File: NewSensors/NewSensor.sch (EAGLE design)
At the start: 9 parts, among them X2 CNY70

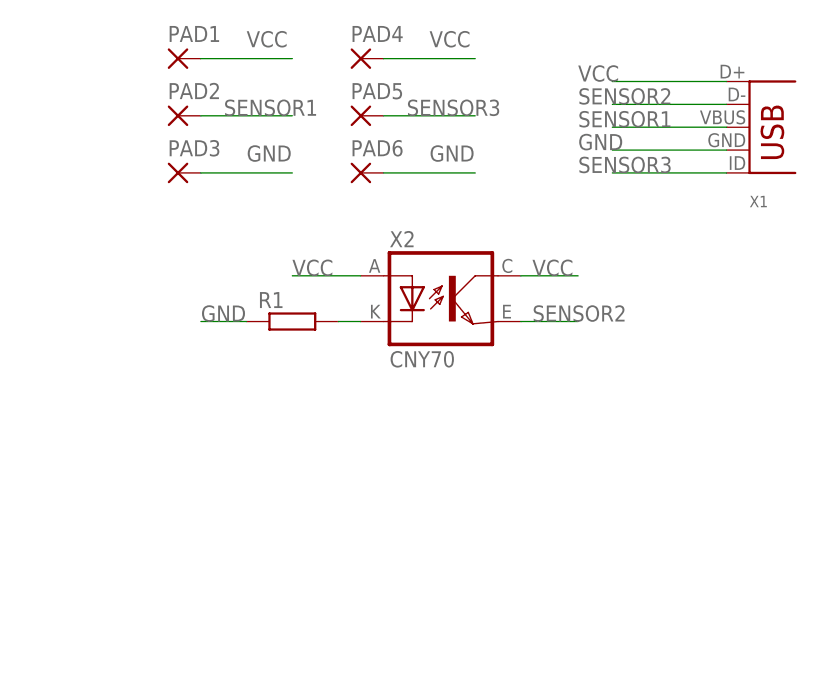
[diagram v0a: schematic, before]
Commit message: Added code V1
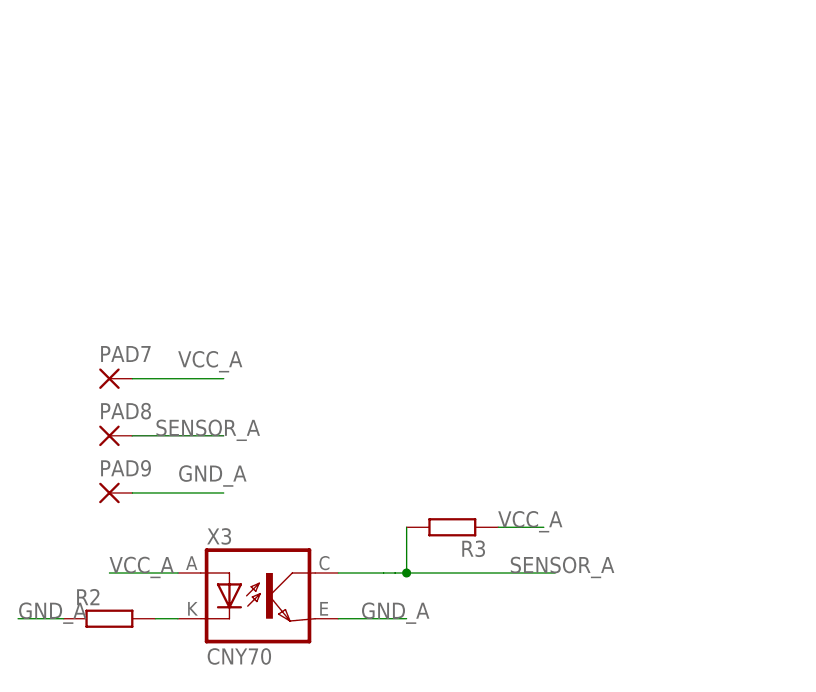
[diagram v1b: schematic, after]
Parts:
- removed PAD1, PAD2, PAD3, PAD4, PAD5, PAD6: WIREPADSMD1,27-254, wirepad:WIREPADSMD1,27-254
- removed R1: (no value), ScyllAlarmV3.0:RCL_R-EU_R0805
- removed X1: (no value), tom:USB-MB-S
- removed X2: CNY70, cny70:CNY70
- added PAD7, PAD8, PAD9: WIREPADSMD1,27-254, wirepad:WIREPADSMD1,27-254
- added R2, R3: (no value), ScyllAlarmV3.0:RCL_R-EU_R0805
- added X3: CNY70, cny70:CNY70
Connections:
- removed net GND: PAD3.P, PAD6.P, R1.1, X1.GND
- removed net N$1: R1.2, X2.C
- removed net SENSOR1: PAD2.P, X1.VBUS
- removed net SENSOR2: X1.D-, X2.EMI
- removed net SENSOR3: PAD5.P, X1.ID
- removed net VCC: PAD1.P, PAD4.P, X1.D+, X2.A, X2.COL
- new net GND_A: PAD9.P, R2.1, X3.EMI
- new net N$2: R2.2, X3.C
- new net SENSOR_A: PAD8.P, R3.2, X3.COL
- new net VCC_A: PAD7.P, R3.1, X3.A
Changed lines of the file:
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@@
 <settings>
 <setting alwaysvectorfont="no"/>
-<setting keepoldvectorfont="yes"/>
 <setting verticaltext="up"/>
 </settings>
@@
 <layer number="88" name="SimResults" color="9" fill="1" visible="yes" active="yes"/>
 <layer number="89" name="SimProbes" color="9" fill="1" visible="yes" active="yes"/>
-<layer number="90" name="Modules" color="5" fill="1" visible="no" active="yes"/>
+<layer number="90" name="Modules" color="5" fill="1" visible="yes" active="yes"/>
 <layer number="91" name="Nets" color="2" fill="1" visible="yes" active="yes"/>
 <layer number="92" name="Busses" color="1" fill="1" visible="yes" active="yes"/>
@@
 </classes>
 <parts>
-<part name="R1" library="ScyllAlarmV3.0" deviceset="RCL_R-EU_" device="R0805"/>
-<part name="X1" library="tom" deviceset="USB" device="-MB-S"/>
-<part name="X2" library="cny70" deviceset="CNY70" device=""/>
-<part name="PAD1" library="wirepad" library_urn="urn:adsk.eagle:library:412" deviceset="WIREPAD" device="SMD1,27-254" package3d_urn="urn:adsk.eagle:package:30839/1" value="WIREPADSMD1,27-254"/>
-<part name="PAD2" library="wirepad" deviceset="WIREPAD" device="SMD1,27-254" value="WIREPADSMD1,27-254"/>
-<part name="PAD3" library="wirepad" deviceset="WIREPAD" device="SMD1,27-254" value="WIREPADSMD1,27-254"/>
-<part name="PAD4" library="wirepad" deviceset="WIREPAD" device="SMD1,27-254" value="WIREPADSMD1,27-254"/>
-<part name="PAD5" library="wirepad" deviceset="WIREPAD" device="SMD1,27-254" value="WIREPADSMD1,27-254"/>
-<part name="PAD6" library="wirepad" deviceset="WIREPAD" device="SMD1,27-254" value="WIREPADSMD1,27-254"/>
+<part name="R2" library="ScyllAlarmV3.0" deviceset="RCL_R-EU_" device="R0805"/>
+<part name="X3" library="cny70" deviceset="CNY70" device=""/>
+<part name="PAD7" library="wirepad" library_urn="urn:adsk.eagle:library:412" deviceset="WIREPAD" device="SMD1,27-254" package3d_urn="urn:adsk.eagle:package:30839/1" value="WIREPADSMD1,27-254"/>
+<part name="PAD8" library="wirepad" deviceset="WIREPAD" device="SMD1,27-254" value="WIREPADSMD1,27-254"/>
+<part name="PAD9" library="wirepad" deviceset="WIREPAD" device="SMD1,27-254" value="WIREPADSMD1,27-254"/>
+<part name="R3" library="ScyllAlarmV3.0" deviceset="RCL_R-EU_" device="R0805"/>
 </parts>
 <sheets>
@@
 </plain>
 <instances>
-<instance part="R1" gate="G$1" x="38.1" y="60.96"/>
-<instance part="X1" gate="G$1" x="88.9" y="78.74"/>
-<instance part="X2" gate="G$1" x="55.88" y="63.5"/>
-<instance part="PAD1" gate="G$1" x="25.4" y="90.17" smashed="yes">
-<attribute name="NAME" x="24.257" y="92.0242" size="1.778" layer="95"/>
+<instance part="R2" gate="G$1" x="17.78" y="27.94"/>
+<instance part="X3" gate="G$1" x="35.56" y="30.48"/>
+<instance part="PAD7" gate="G$1" x="17.78" y="54.61" smashed="yes">
+<attribute name="NAME" x="16.637" y="56.4642" size="1.778" layer="95"/>
 </instance>
-<instance part="PAD2" gate="G$1" x="25.4" y="83.82" smashed="yes">
-<attribute name="NAME" x="24.257" y="85.6742" size="1.778" layer="95"/>
+<instance part="PAD8" gate="G$1" x="17.78" y="48.26" smashed="yes">
+<attribute name="NAME" x="16.637" y="50.1142" size="1.778" layer="95"/>
 </instance>
-<instance part="PAD3" gate="G$1" x="25.4" y="77.47" smashed="yes">
-<attribute name="NAME" x="24.257" y="79.3242" size="1.778" layer="95"/>
+<instance part="PAD9" gate="G$1" x="17.78" y="41.91" smashed="yes">
+<attribute name="NAME" x="16.637" y="43.7642" size="1.778" layer="95"/>
 </instance>
-<instance part="PAD4" gate="G$1" x="45.72" y="90.17" smashed="yes">
-<attribute name="NAME" x="44.577" y="92.0242" size="1.778" layer="95"/>
-</instance>
-<instance part="PAD5" gate="G$1" x="45.72" y="83.82" smashed="yes">
-<attribute name="NAME" x="44.577" y="85.6742" size="1.778" layer="95"/>
-</instance>
-<instance part="PAD6" gate="G$1" x="45.72" y="77.47" smashed="yes">
-<attribute name="NAME" x="44.577" y="79.3242" size="1.778" layer="95"/>
-</instance>
+<instance part="R3" gate="G$1" x="55.88" y="38.1" rot="R180"/>
 </instances>
 <busses>
 </busses>
 <nets>
-<net name="SENSOR1" class="0">
-<segment>
-<pinref part="PAD2" gate="G$1" pin="P"/>
-<wire x1="27.94" y1="83.82" x2="38.1" y2="83.82" width="0.1524" layer="91"/>
-<label x="30.48" y="83.82" size="1.778" layer="95"/>
-</segment>
-<segment>
-<pinref part="X1" gate="G$1" pin="VBUS"/>
-<wire x1="86.36" y1="82.55" x2="73.66" y2="82.55" width="0.1524" layer="91"/>
-<label x="69.85" y="82.55" size="1.778" layer="95"/>
-</segment>
-</net>
-<net name="SENSOR2" class="0">
-<segment>
-<pinref part="X2" gate="G$1" pin="EMI"/>
-<wire x1="63.5" y1="60.96" x2="69.85" y2="60.96" width="0.1524" layer="91"/>
-<label x="64.77" y="60.96" size="1.778" layer="95"/>
-</segment>
-<segment>
-<pinref part="X1" gate="G$1" pin="D-"/>
-<wire x1="86.36" y1="85.09" x2="73.66" y2="85.09" width="0.1524" layer="91"/>
-<label x="69.85" y="85.09" size="1.778" layer="95"/>
-</segment>
-</net>
-<net name="SENSOR3" class="0">
-<segment>
-<pinref part="X1" gate="G$1" pin="ID"/>
-<wire x1="86.36" y1="77.47" x2="73.66" y2="77.47" width="0.1524" layer="91"/>
-<label x="69.85" y="77.47" size="1.778" layer="95"/>
-</segment>
-<segment>
-<pinref part="PAD5" gate="G$1" pin="P"/>
-<wire x1="48.26" y1="83.82" x2="58.42" y2="83.82" width="0.1524" layer="91"/>
-<label x="50.8" y="83.82" size="1.778" layer="95"/>
-</segment>
-</net>
-<net name="VCC" class="0">
-<segment>
-<pinref part="X2" gate="G$1" pin="A"/>
-<wire x1="45.72" y1="66.04" x2="38.1" y2="66.04" width="0.1524" layer="91"/>
-<label x="38.1" y="66.04" size="1.778" layer="95"/>
-</segment>
-<segment>
-<pinref part="X2" gate="G$1" pin="COL"/>
-<wire x1="63.5" y1="66.04" x2="69.85" y2="66.04" width="0.1524" layer="91"/>
-<label x="64.77" y="66.04" size="1.778" layer="95"/>
-</segment>
-<segment>
-<pinref part="PAD1" gate="G$1" pin="P"/>
-<wire x1="27.94" y1="90.17" x2="38.1" y2="90.17" width="0.1524" layer="91"/>
-<label x="33.02" y="91.44" size="1.778" layer="95"/>
-</segment>
-<segment>
-<pinref part="PAD4" gate="G$1" pin="P"/>
-<wire x1="48.26" y1="90.17" x2="58.42" y2="90.17" width="0.1524" layer="91"/>
-<label x="53.34" y="91.44" size="1.778" layer="95"/>
-</segment>
-<segment>
-<pinref part="X1" gate="G$1" pin="D+"/>
-<wire x1="86.36" y1="87.63" x2="73.66" y2="87.63" width="0.1524" layer="91"/>
-<label x="69.85" y="87.63" size="1.778" layer="95"/>
-</segment>
-</net>
-<net name="GND" class="0">
-<segment>
-<pinref part="X1" gate="G$1" pin="GND"/>
-<wire x1="86.36" y1="80.01" x2="73.66" y2="80.01" width="0.1524" layer="91"/>
-<label x="69.85" y="80.01" size="1.778" layer="95"/>
-</segment>
-<segment>
-<pinref part="R1" gate="G$1" pin="1"/>
-<wire x1="33.02" y1="60.96" x2="27.94" y2="60.96" width="0.1524" layer="91"/>
-<label x="27.94" y="60.96" size="1.778" layer="95"/>
-</segment>
-<segment>
-<pinref part="PAD3" gate="G$1" pin="P"/>
-<wire x1="27.94" y1="77.47" x2="38.1" y2="77.47" width="0.1524" layer="91"/>
-<label x="33.02" y="78.74" size="1.778" layer="95"/>
-</segment>
-<segment>
-<pinref part="PAD6" gate="G$1" pin="P"/>
-<wire x1="48.26" y1="77.47" x2="58.42" y2="77.47" width="0.1524" layer="91"/>
-<label x="53.34" y="78.74" size="1.778" layer="95"/>
-</segment>
-</net>
-<net name="N$1" class="0">
-<segment>
-<pinref part="R1" gate="G$1" pin="2"/>
-<pinref part="X2" gate="G$1" pin="C"/>
-<wire x1="43.18" y1="60.96" x2="45.72" y2="60.96" width="0.1524" layer="91"/>
-</segment>
-</net>
+<net name="N$2" class="0">
+<segment>
+<pinref part="R2" gate="G$1" pin="2"/>
+<pinref part="X3" gate="G$1" pin="C"/>
+<wire x1="22.86" y1="27.94" x2="25.4" y2="27.94" width="0.1524" layer="91"/>
+</segment>
+</net>
+<net name="VCC_A" class="0">
+<segment>
+<pinref part="PAD7" gate="G$1" pin="P"/>
+<wire x1="20.32" y1="54.61" x2="30.48" y2="54.61" width="0.1524" layer="91"/>
+<label x="25.4" y="55.88" size="1.778" layer="95"/>
+</segment>
+<segment>
+<pinref part="X3" gate="G$1" pin="A"/>
+<wire x1="25.4" y1="33.02" x2="17.78" y2="33.02" width="0.1524" layer="91"/>
+<label x="17.78" y="33.02" size="1.778" layer="95"/>
+</segment>
+<segment>
+<pinref part="R3" gate="G$1" pin="1"/>
+<wire x1="60.96" y1="38.1" x2="66.04" y2="38.1" width="0.1524" layer="91"/>
+<label x="60.96" y="38.1" size="1.778" layer="95"/>
+</segment>
+</net>
+<net name="SENSOR_A" class="0">
+<segment>
+<pinref part="PAD8" gate="G$1" pin="P"/>
+<wire x1="20.32" y1="48.26" x2="30.48" y2="48.26" width="0.1524" layer="91"/>
+<label x="22.86" y="48.26" size="1.778" layer="95"/>
+</segment>
+<segment>
+<label x="62.23" y="33.02" size="1.778" layer="95"/>
+<pinref part="R3" gate="G$1" pin="2"/>
+<wire x1="50.8" y1="33.02" x2="67.31" y2="33.02" width="0.1524" layer="91"/>
+<wire x1="50.8" y1="38.1" x2="50.8" y2="33.02" width="0.1524" layer="91"/>
+<wire x1="43.18" y1="33.02" x2="48.26" y2="33.02" width="0.1524" layer="91"/>
+<wire x1="48.26" y1="33.02" x2="49.53" y2="33.02" width="0.1524" layer="91"/>
+<wire x1="50.8" y1="33.02" x2="49.53" y2="33.02" width="0.1524" layer="91"/>
+<junction x="50.8" y="33.02"/>
+<pinref part="X3" gate="G$1" pin="COL"/>
+</segment>
+</net>
+<net name="GND_A" class="0">
+<segment>
+<pinref part="PAD9" gate="G$1" pin="P"/>
+<wire x1="20.32" y1="41.91" x2="30.48" y2="41.91" width="0.1524" layer="91"/>
+<label x="25.4" y="43.18" size="1.778" layer="95"/>
+</segment>
+<segment>
+<pinref part="R2" gate="G$1" pin="1"/>
+<wire x1="12.7" y1="27.94" x2="7.62" y2="27.94" width="0.1524" layer="91"/>
+<label x="7.62" y="27.94" size="1.778" layer="95"/>
+</segment>
+<segment>
+<wire x1="43.18" y1="27.94" x2="50.8" y2="27.94" width="0.1524" layer="91"/>
+<label x="45.72" y="27.94" size="1.778" layer="95"/>
+<pinref part="X3" gate="G$1" pin="EMI"/>
+</segment>
+</net>
